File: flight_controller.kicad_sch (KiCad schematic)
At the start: 46 parts, among them IC1 BQ25883, IC2 STM32F722RET6, J1 Screw_Terminal_01x02, J3 USB-C, J4 MicroSD Socket, U1 BMP581, U2 TPS630702RNMR

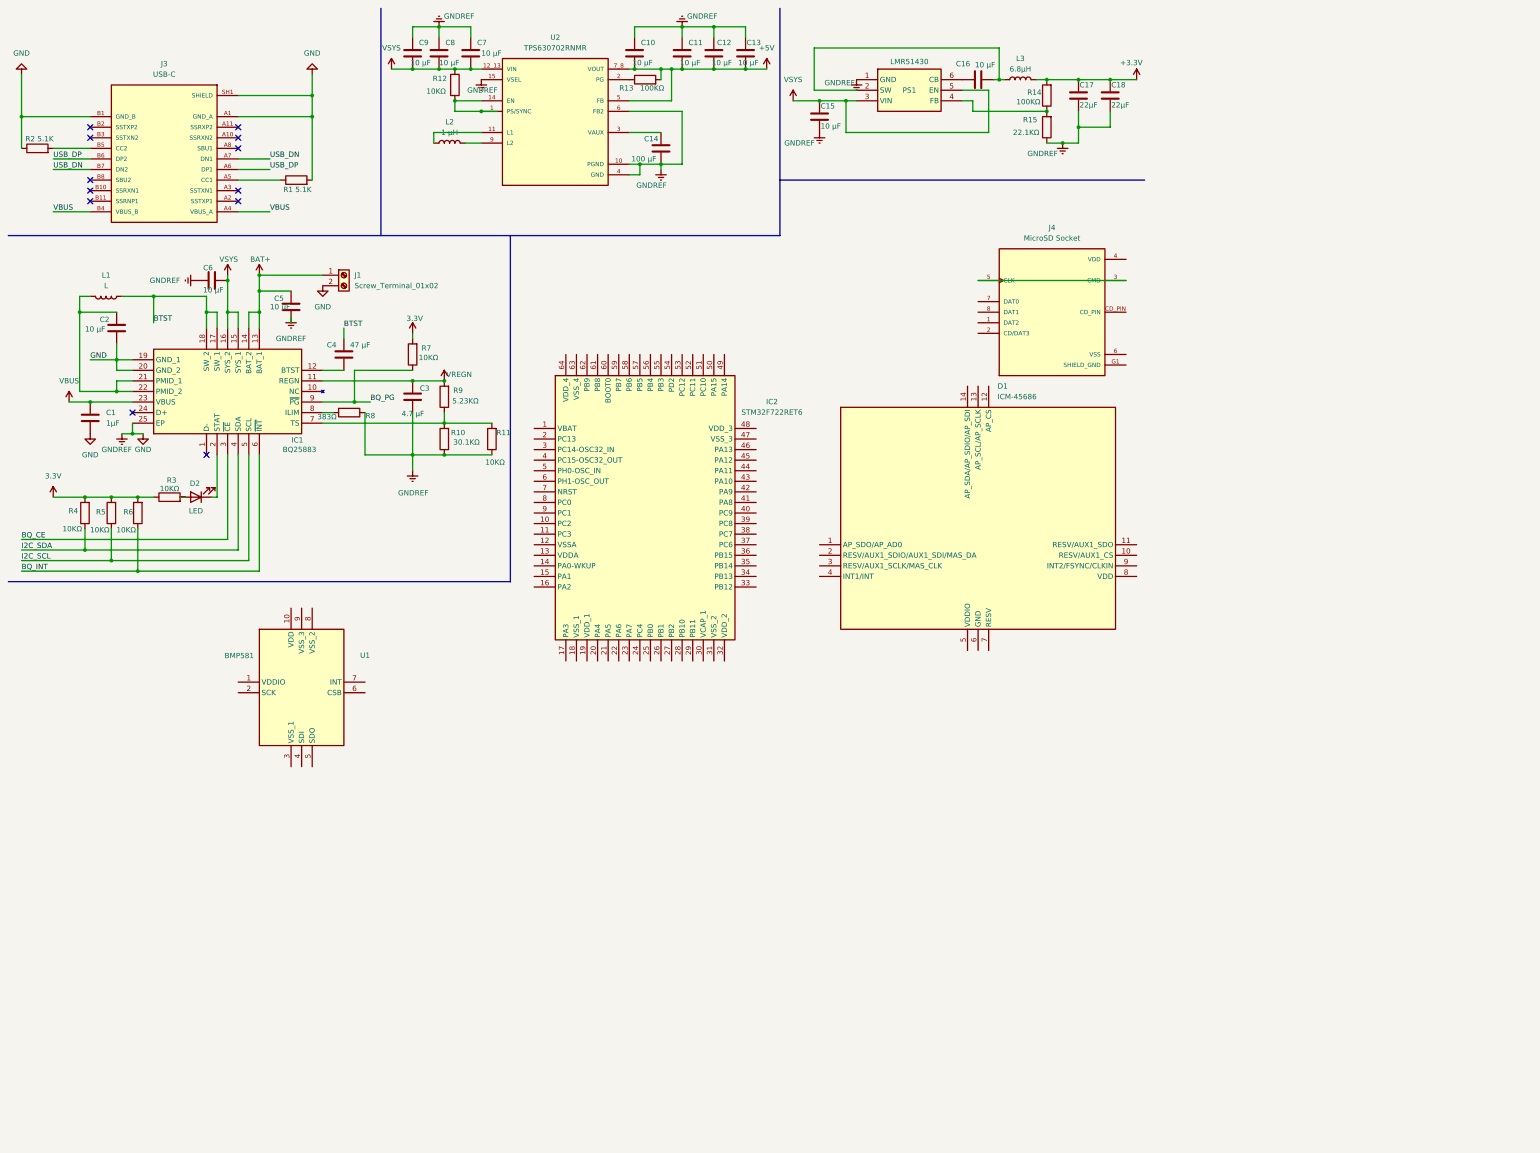
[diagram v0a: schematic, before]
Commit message: electric schematic
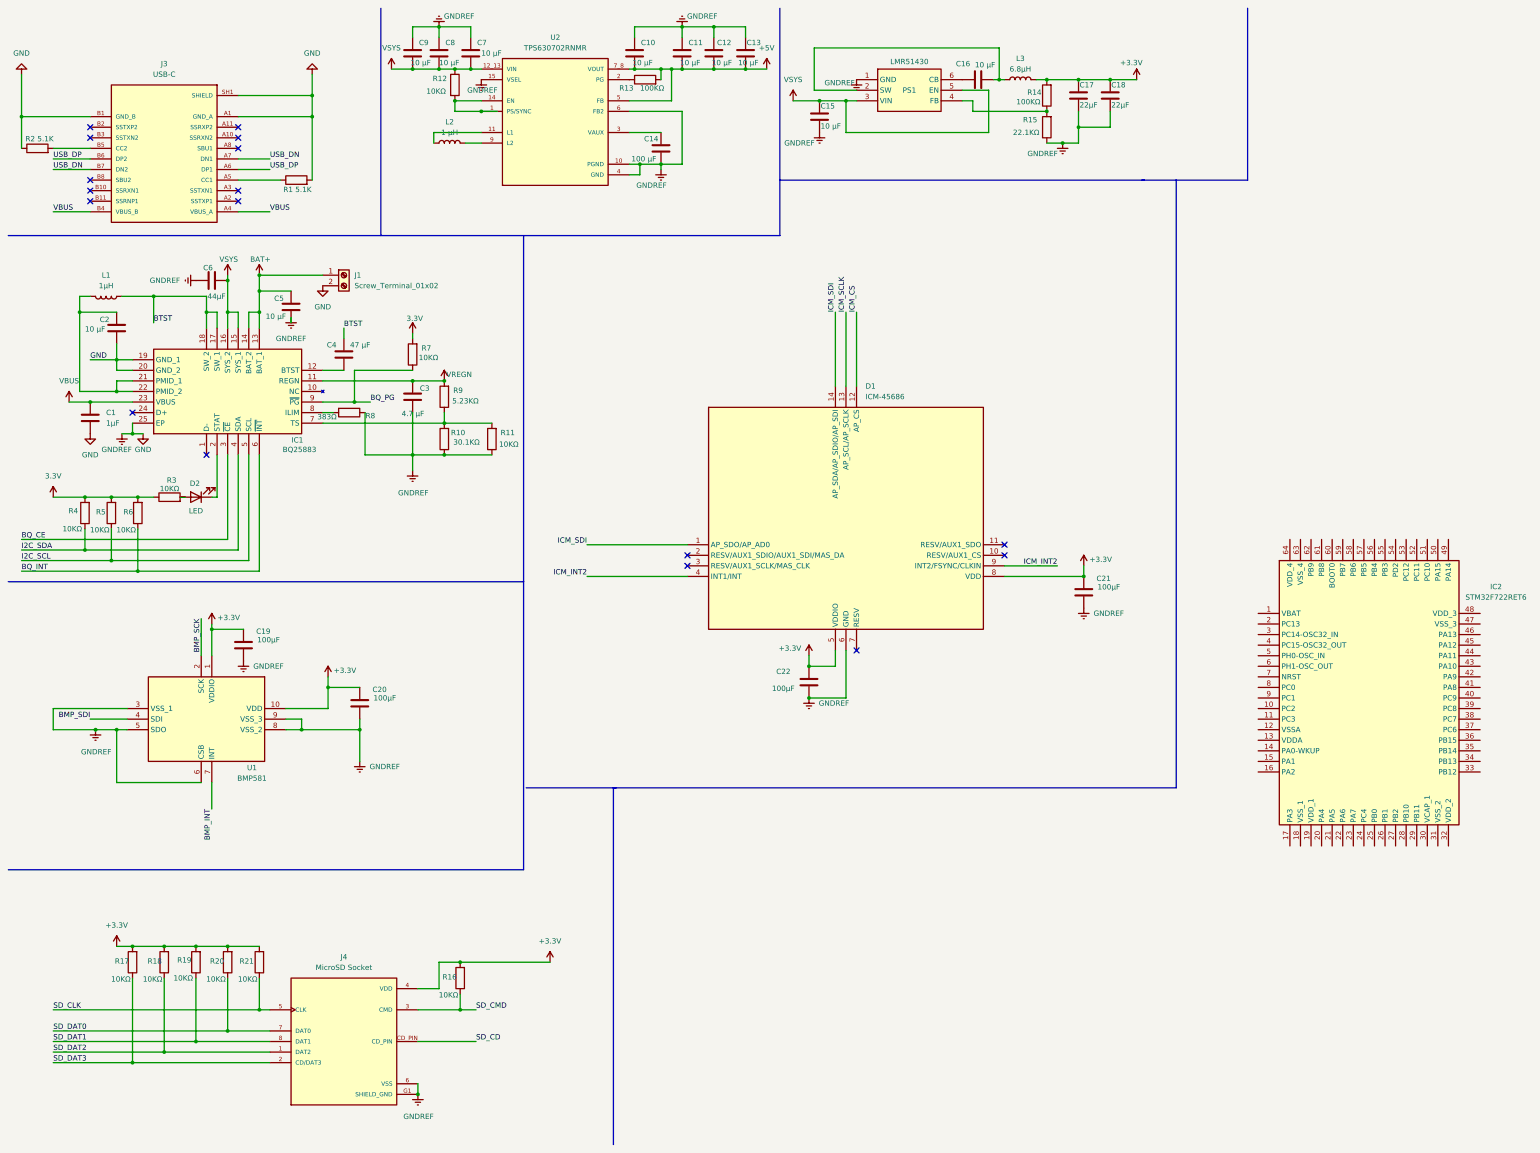
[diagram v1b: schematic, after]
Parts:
- added C19, C20, C21, C22: 100μF, symbol Device:C
- added R16, R17, R18, R19, R20, R21: 10KΩ, symbol Device:R
- C6: value 10 μF -> 44μF
- L1: value L -> 1μH
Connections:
- net SHIELD_GND is gone; now on net GND: J4.G1 (SHIELD_GND), J4.G2 (SHIELD_GND), J4.G3 (SHIELD_GND)
- net +3.3V: now also D1.5 (VDDIO), D1.8 (VDD), J4.4 (VDD), U1.1 (VDDIO), U1.10 (VDD), C19.1, C20.1, C21.1, C22.1, R16.2, R17.2, R18.2, R19.2, R20.2, R21.2
- net GND: now also D1.6 (GND), J4.6 (VSS), U1.3 (VSS_1), U1.5 (SDO), U1.6 (CSB), U1.8 (VSS_2), U1.9 (VSS_3), C19.2, C20.2, C21.2, C22.2
- net BMP_SCK: now reaches U1.2 (SCK)
- net BMP_SDI: now reaches U1.4 (SDI)
- net BMP_INT: now reaches U1.7 (INT)
- net ICM_SDI: now reaches D1.1 (AP_SDO/AP_AD0)
- net ICM_SDI: now also D1.14 (AP_SDA/AP_SDIO/AP_SDI)
- net ICM_CS: now reaches D1.12 (AP_CS)
- net ICM_SCLK: now reaches D1.13 (AP_SCL/AP_SCLK)
- net ICM_INT2: now reaches D1.4 (INT1/INT)
- net ICM_INT2: now also D1.9 (INT2/FSYNC/CLKIN)
- net SD_DAT2: now reaches J4.1 (DAT2)
- net SD_DAT2: now also R18.1
- net SD_DAT3: now reaches J4.2 (CD/DAT3)
- net SD_DAT3: now also R17.1
- net SD_CLK: now reaches J4.5 (CLK)
- net SD_CLK: now also R21.1; no longer J4.3 (CMD)
- net SD_DAT0: now reaches J4.7 (DAT0)
- net SD_DAT0: now also R20.1
- net SD_DAT1: now reaches J4.8 (DAT1)
- net SD_DAT1: now also R19.1
- net SD_CD: now reaches J4.CD_PIN
- new net SD_CMD: J4.3 (CMD), R16.1
- no-connect marks 12 -> 17
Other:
- moved on the sheet: D1, IC2, J4, U1
